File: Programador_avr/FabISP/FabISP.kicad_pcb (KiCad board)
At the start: 2 copper layers, 41 x 19 mm, 14 parts, among them IC1 ATTINY44, M1 Reson., M2 PINHD-1x02-SMD-HEADER, M3 MICRO-USB, M4 PINHD-1x02-SMD-HEADER

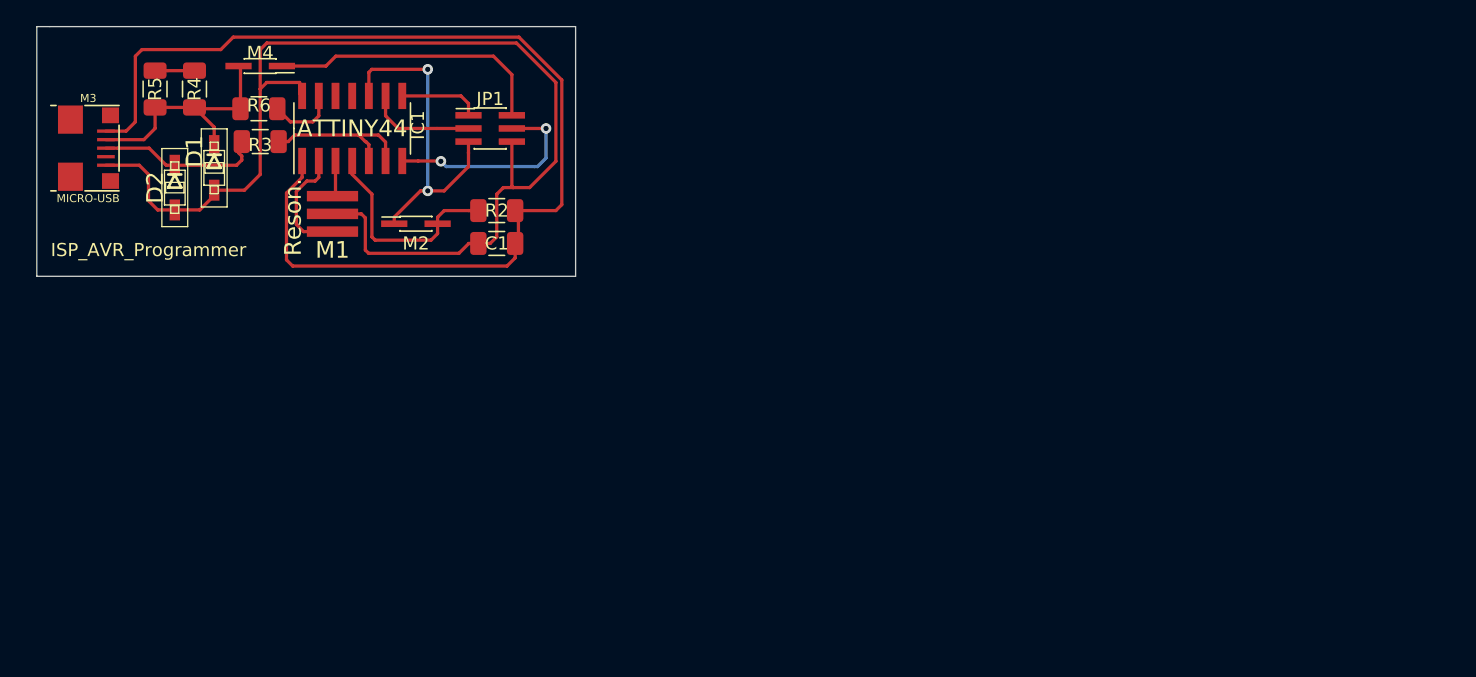
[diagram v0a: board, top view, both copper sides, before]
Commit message: Generación de BOM y gerbers
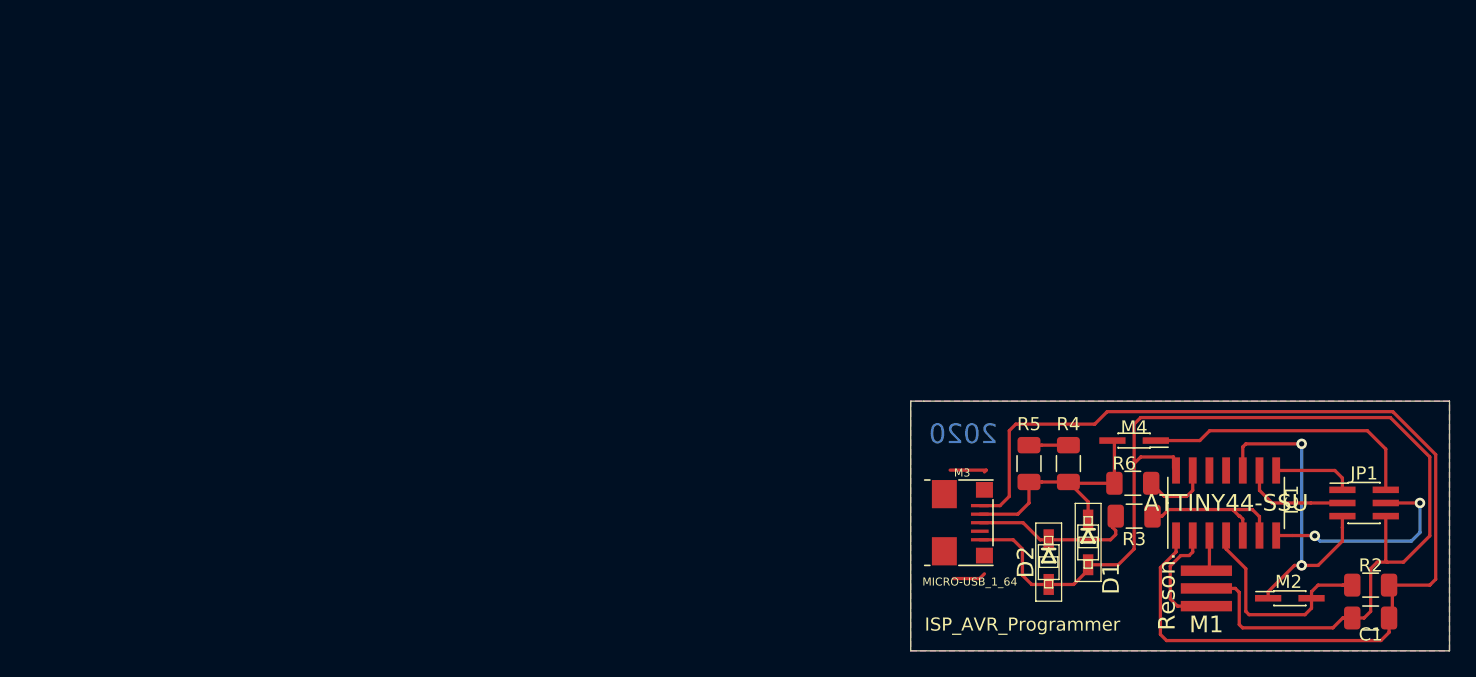
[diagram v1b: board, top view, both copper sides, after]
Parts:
- IC1: value ATTINY44 -> ATTINY44-SSU
- M3: value MICRO-USB -> MICRO-USB_1_64
- moved C1 72.3 mm to (160.5, 104.0)
- moved D1 72.3 mm to (139.0, 98.2)
- moved D2 72.3 mm to (136.0, 99.8)
- moved IC1 72.3 mm to (149.5, 95.2)
- moved JP1 72.3 mm to (160.0, 95.2)
- moved M1 72.3 mm to (148.0, 101.8)
- moved M2 72.3 mm to (154.3, 102.5)
- moved M3 72.3 mm to (129.2, 96.8)
- moved M4 72.3 mm to (142.5, 90.5)
- moved R2 72.3 mm to (160.5, 101.5)
- moved R3 72.3 mm to (142.5, 96.2)
- moved R4 72.3 mm to (134.5, 92.2)
- moved R5 72.3 mm to (137.5, 92.2)
- moved R6 72.3 mm to (142.4, 93.8)
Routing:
- net (no net): track 0.00 -> 5.46 mm
- added copper zone on B.Cu, net (none)
- added copper zone on F.Cu, net (none)
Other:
- board text added: "2020"
